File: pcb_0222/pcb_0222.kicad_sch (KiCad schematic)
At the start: 52 parts

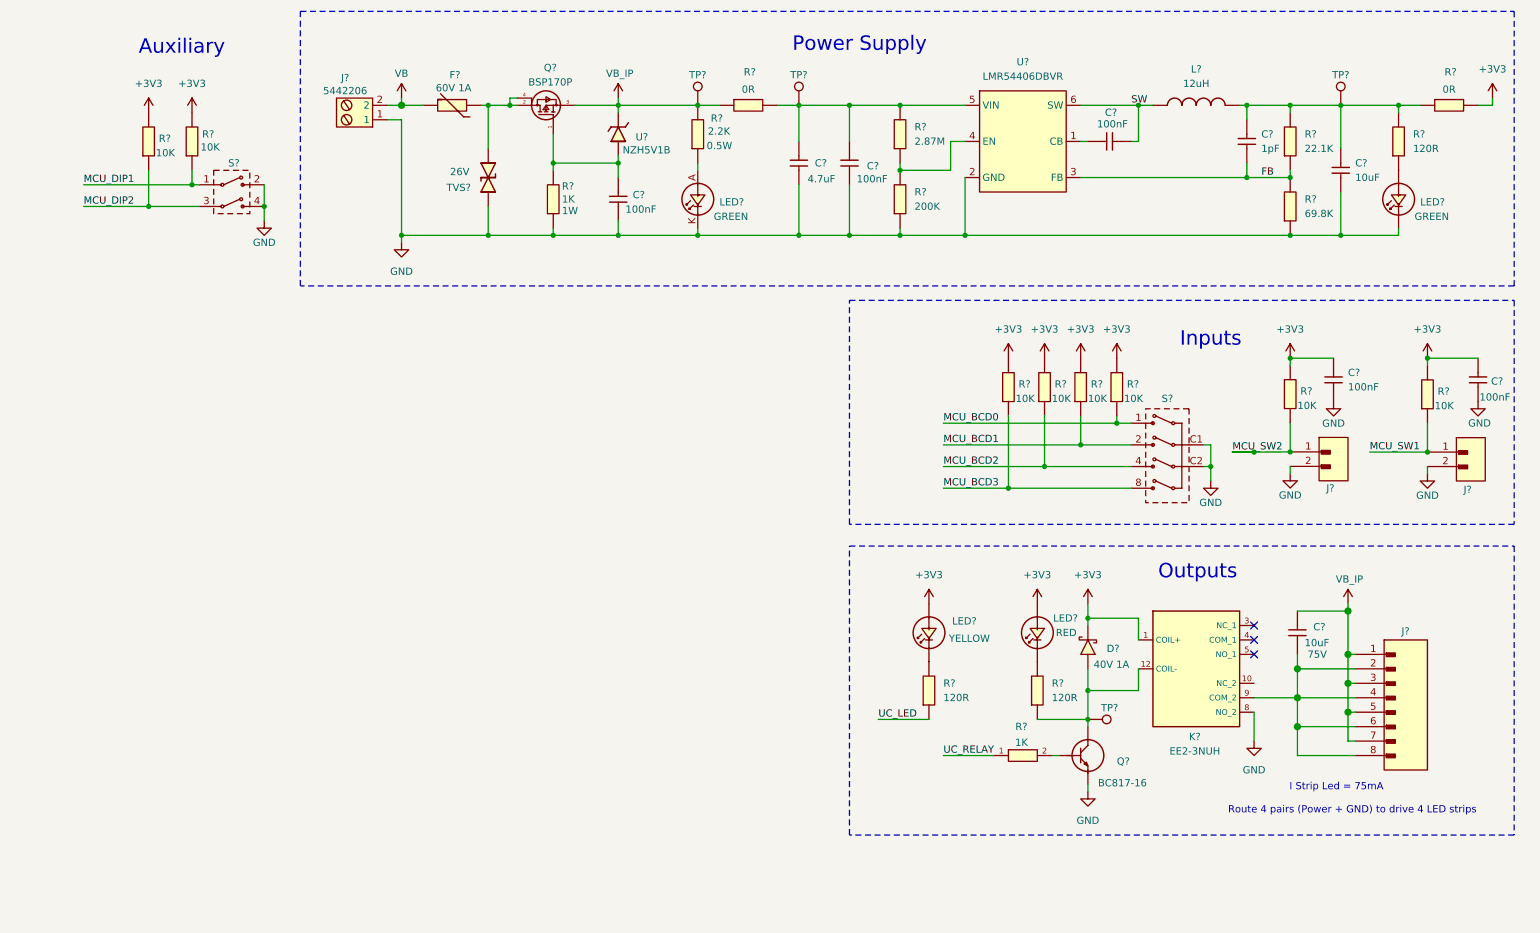
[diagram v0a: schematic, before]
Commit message: Schematic On Review
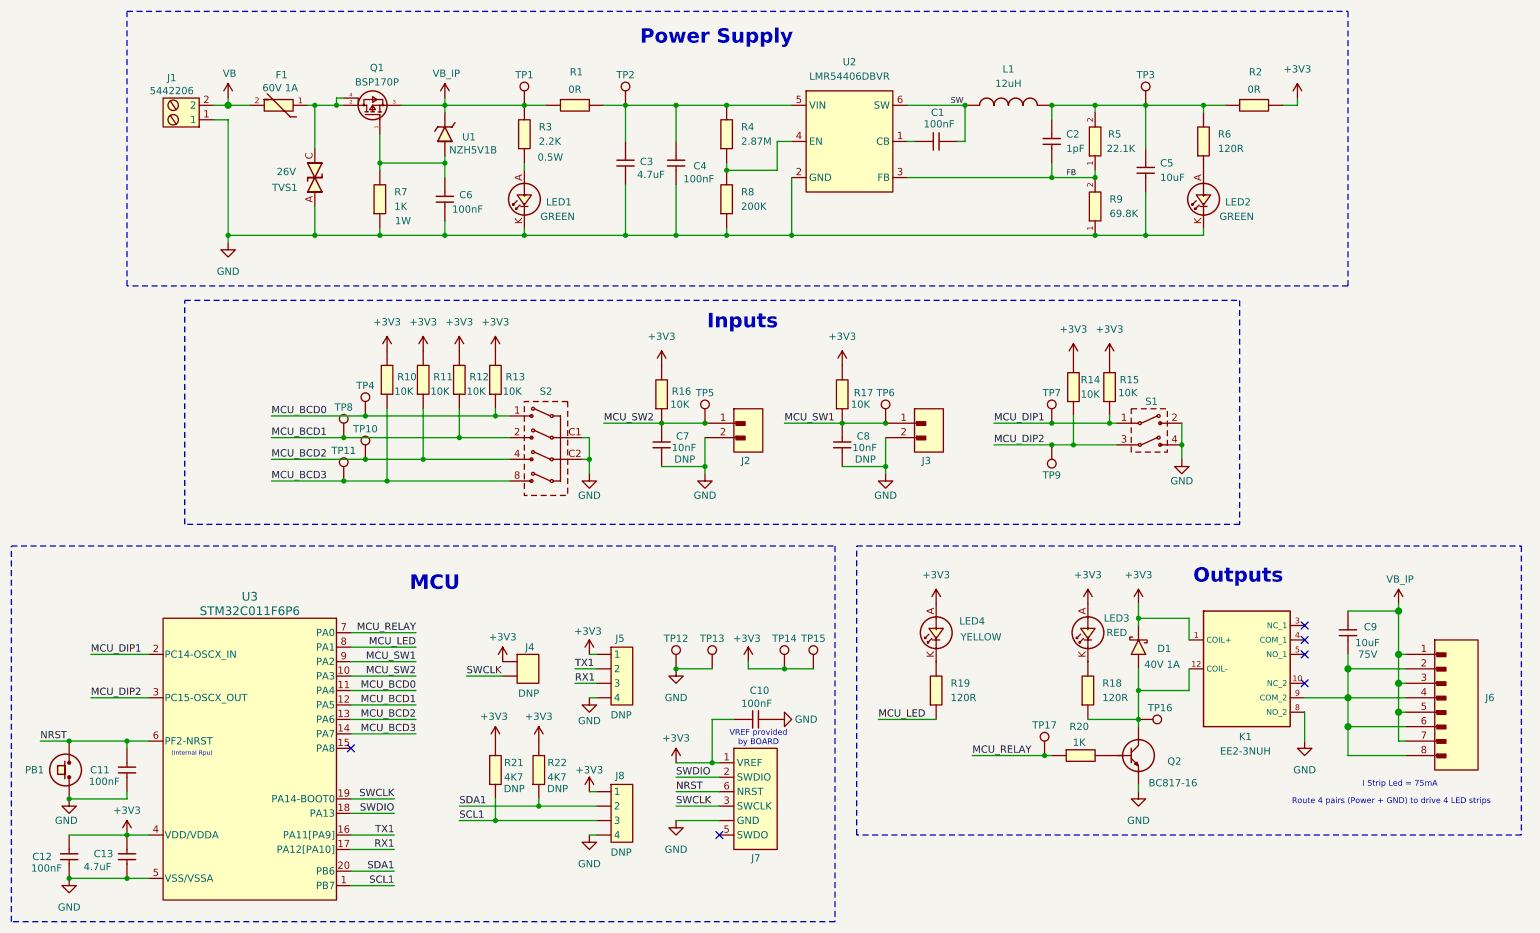
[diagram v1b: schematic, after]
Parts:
- removed C?: 4.7uF, passives_smd:C_1206_h1.8mm, symbol C_capacitors_ceramic:C_1206_4.7uF_50V_X7R
- removed C? (x2): 100nF, passives_smd:C_0603, symbol C_capacitors_ceramic:C_0603_100nF_50V
- removed C?: 1pF, passives_smd:C_0603, symbol C_capacitors_ceramic:C_0603_1pF_50V
- removed J?: SM08B-PASS-TBT, symbol J_connectors_headers:SM08B-PASS-TBT
- removed J?: SM02B-PASS-TBT, symbol J_connectors_headers:SM02B-PASS-TBT
- removed L?: 12uH, symbol L_inductors:L_6.8x6.8mm_12uH_1.7A
- removed R?: 200K, passives_smd:R_0603, symbol R_resistors:R_0603_200K_1%
- removed R?: 2.2K, passives_smd:R_1206, symbol R_resistors:R_1206_2K7_1%_500mW
- removed R?: 22.1K, passives_smd:R_0603, symbol R_resistors:R_0603_22.1K_1%
- removed R?: 1K, symbol R_resistors:R_2512_1K_1%_1W_AEC_Q200
- removed R?: 2.87M, passives_smd:R_0603, symbol R_resistors:R_0603_2.87M_1%
- removed R?: 0R, passives_smd:R_0603, symbol R_resistors:R_0603_0R
- removed R?: 10K, passives_smd:R_0603, symbol R_resistors:R_0603_10K_1%
- removed TP?: (no value), testpoints:TP_SMD_2mm, symbol TP_testpoints:TP_SMD_2MM
- added C10, C11, C12: 100nF, passives_smd:C_0603, symbol C_capacitors_ceramic:C_0603_100nF_50V
- added C13: 4.7uF, passives_smd:C_0603, symbol C_capacitors_ceramic:C_0603_4.7uF_10V
- added C2: 1pF, passives_smd:C_0603, symbol C_capacitors_ceramic:C_0603_1pF_50V_C0G
- added C3: 4.7uF, passives_smd:C_0603, symbol C_capacitors_ceramic:C_0603_4.7uF_35V
- added C7, C8: 10nF, passives_smd:C_0603, symbol C_capacitors_ceramic:C_0603_10nF_50V
- added J2: SM02B-PASS-TBT, symbol J_connectors_headers:SM02B-PASS-TBT
- added J4: HEADER_MALE_THT_0.1"_2x1, connectors_headers:77311-118-02LF, symbol J_connectors_headers:HEADER_MALE_THT_0.1{dblquote}_2x1
- added J5, J8: HEADER_MALE_THT_0.1"_4x1, symbol J_connectors_headers:HEADER_MALE_THT_0.1{dblquote}_4x1
- added J6: SM08B-PASS-TBT, symbol J_connectors_headers:SM08B-PASS-TBT
- added J7: TC-2030-IDC, symbol J_connectors_prog:TC-2030-IDC
- added L1: 12uH, symbol L_inductors:L_44.88mm3_6.8x6.8mm_12uH_1.7A
- added PB1: (no value), switches_smd:7914J-1-000, symbol S_switches_pushbutton:7914J-1-000
- added R1: 0R, passives_smd:R_0603, symbol R_resistors:R_0603_0R
- added R16: 10K, passives_smd:R_0603, symbol R_resistors:R_0603_10K_1%
- added R21, R22: 4K7, passives_smd:R_0603, symbol R_resistors:R_0603_4K7_1%
- added R3: 2.2K, passives_smd:R_1206, symbol R_resistors:R_1206_2.2K_0.5W
- added R4: 2.87M, passives_smd:R_0603, symbol R_resistors:R_0603_2.87M_1%_0.1W
- added R5: 22.1K, passives_smd:R_0603, symbol R_resistors:R_0603_22.1K_1%
- added R7: 1K, passives_smd:R_2512, symbol R_resistors:R_2512_1K_1%_1W_AEC-Q200
- added R8: 200K, passives_smd:R_0603, symbol R_resistors:R_0603_200K_1%_0.1W
- added TP1, TP10, TP11, TP12, TP13, TP14, TP15, TP17, TP4, TP5, TP6, TP7, TP8, TP9: (no value), testpoints:TP_SMD_2mm, symbol TP_testpoints:TP_SMD_2MM
- added U3: STM32C011F6P6, symbol U_microcontrollers:STM32C011F6P6
- C1, C4, C6: renamed from C?; TEMP. COEFF. (none) -> X7R; TOLERANCE (none) -> 10%; VOLTAGE (none) -> 50V
- R18, R19, R6: renamed from R?; PWR (none) -> 1/10W; TEMP. COEFF. (none) -> ±100ppm/°C; TOLERANCE (none) -> 1%
- gave numbers to parts that had none: 31
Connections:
- net +3V3: now also C10.2, C12.2, C13.2, J4.1, J5.1, J7.1 (VREF), J8.1, R16.2, R21.2, R22.2, TP14.1, TP15.1, U3.4 (VDD/VDDA)
- net FB: now also C2.1, R5.1
- net GND: now also C10.1, C11.1, C12.1, C13.1, C3.1, C7.1, C8.1, J2.2, J5.4, J7. (GND), J8.4, PB1.1, PB1.2, R7.1, R8.1, TP12.1, TP13.1, U3.5 (VSS/VSSA)
- net MCU_BCD0: now also TP4.1, U3.11 (PA4)
- net MCU_BCD1: now also TP8.1, U3.12 (PA5)
- net MCU_BCD2: now also TP10.1, U3.13 (PA6)
- net MCU_BCD3: now also TP11.1, U3.14 (PA7)
- net MCU_DIP1: now also TP7.1, U3.2 (PC14-OSCX_IN)
- net MCU_DIP2: now also TP9.1, U3.3 (PC15-OSCX_OUT)
- net MCU_SW1: now also C8.2, TP6.1, U3.9 (PA2)
- net MCU_SW2: now also C7.2, J2.1, R16.1, TP5.1, U3.10 (PA3)
- net SW: now also L1.1
- net VB_IP: now also J6.1, J6.3, J6.5, J6.7, R1.1, R3.2, TP1.1; no longer TP2.1
- net at C6.2, Q1.1, U1.A: now also R7.2
- net at C9.1, K1.9 (COM_2): now also J6.2, J6.4, J6.6, J6.8
- net at U2.4 (EN): now also R4.1, R8.2
- net at C5.2, R2.1, R6.2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: now also C2.2, L1.2, R5.2
- net at LED1.A: now also R3.1
- net at C4.2, U2.5 (VIN): now also TP2.1, C3.2, R1.2, R4.2
- net UC_LED renamed MCU_LED
- net MCU_LED: now also U3.8 (PA1)
- net UC_RELAY renamed MCU_RELAY
- net MCU_RELAY: now also TP17.1, U3.7 (PA0)
- new net NRST: C11.2, J7.6 (NRST), PB1.3, PB1.4, U3.6 (PF2-NRST)
- new net RX1: J5.3, U3.17 (PA12[PA10])
- new net SCL1: J8.3, R21.1, U3.1 (PB7)
- new net SDA1: J8.2, R22.1, U3.20 (PB6)
- new net SWCLK: J4.2, J7.3 (SWCLK), U3.19 (PA14-BOOT0)
- new net SWDIO: J7.2 (SWDIO), U3.18 (PA13)
- new net TX1: J5.2, U3.16 (PA11[PA9])
- no-connect marks 3 -> 6
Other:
- note added: "(Internal Rpu)"
- note added: "MCU"
- note added: "VREF provided by BOARD"
- note removed: "Auxiliary"
- moved on the sheet: C1, C4, C5, C6, C9, D1, J1, J3, K1, LED1, Q1, Q2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
